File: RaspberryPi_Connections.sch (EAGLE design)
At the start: 4 parts

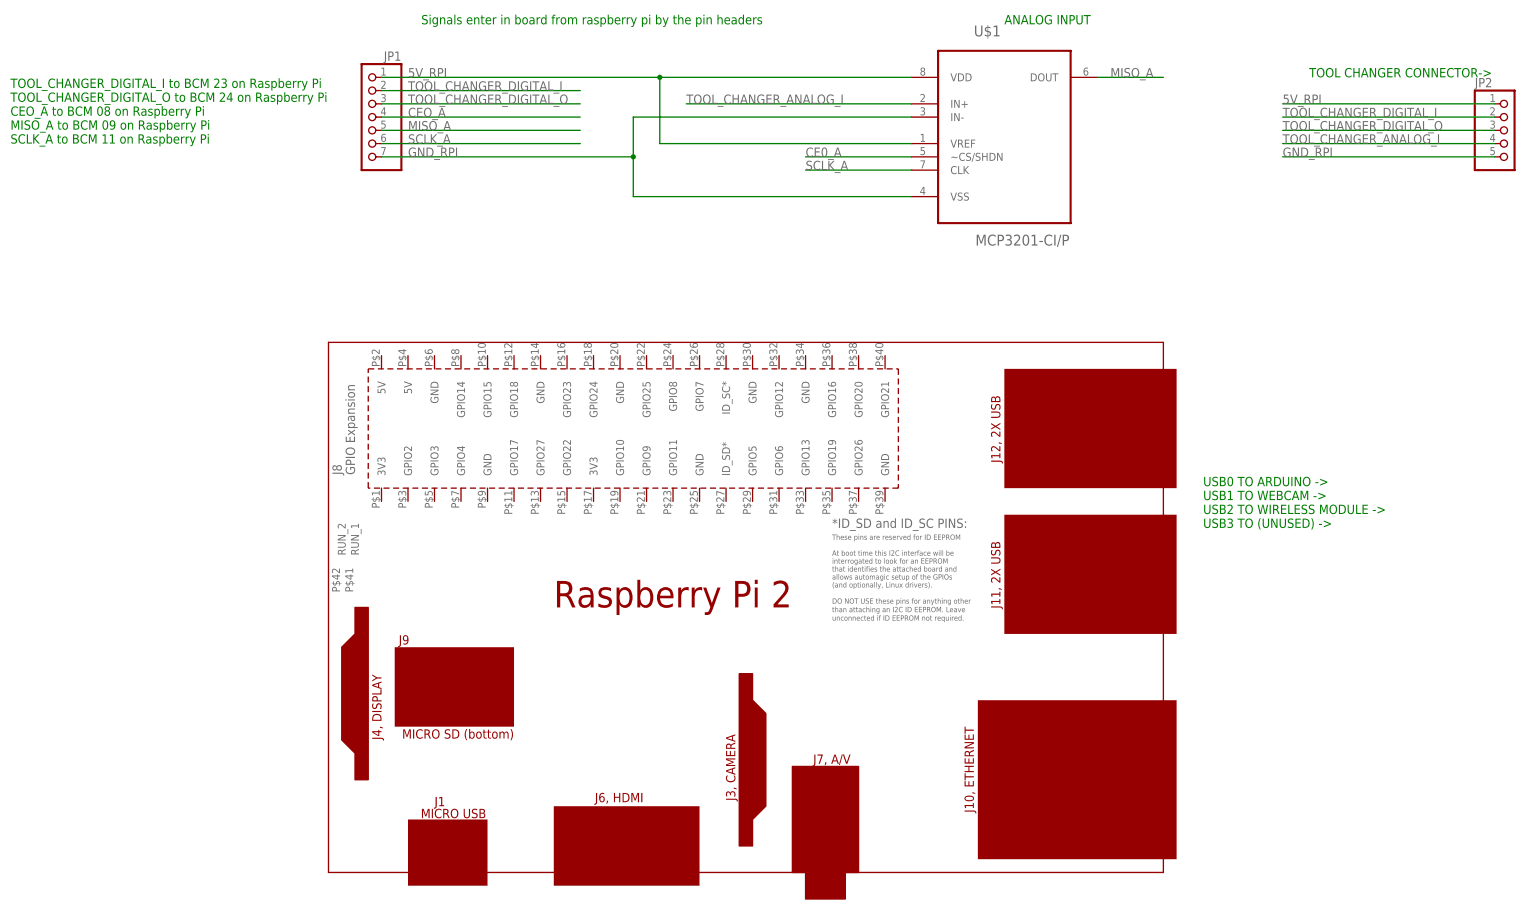
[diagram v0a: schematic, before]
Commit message: update
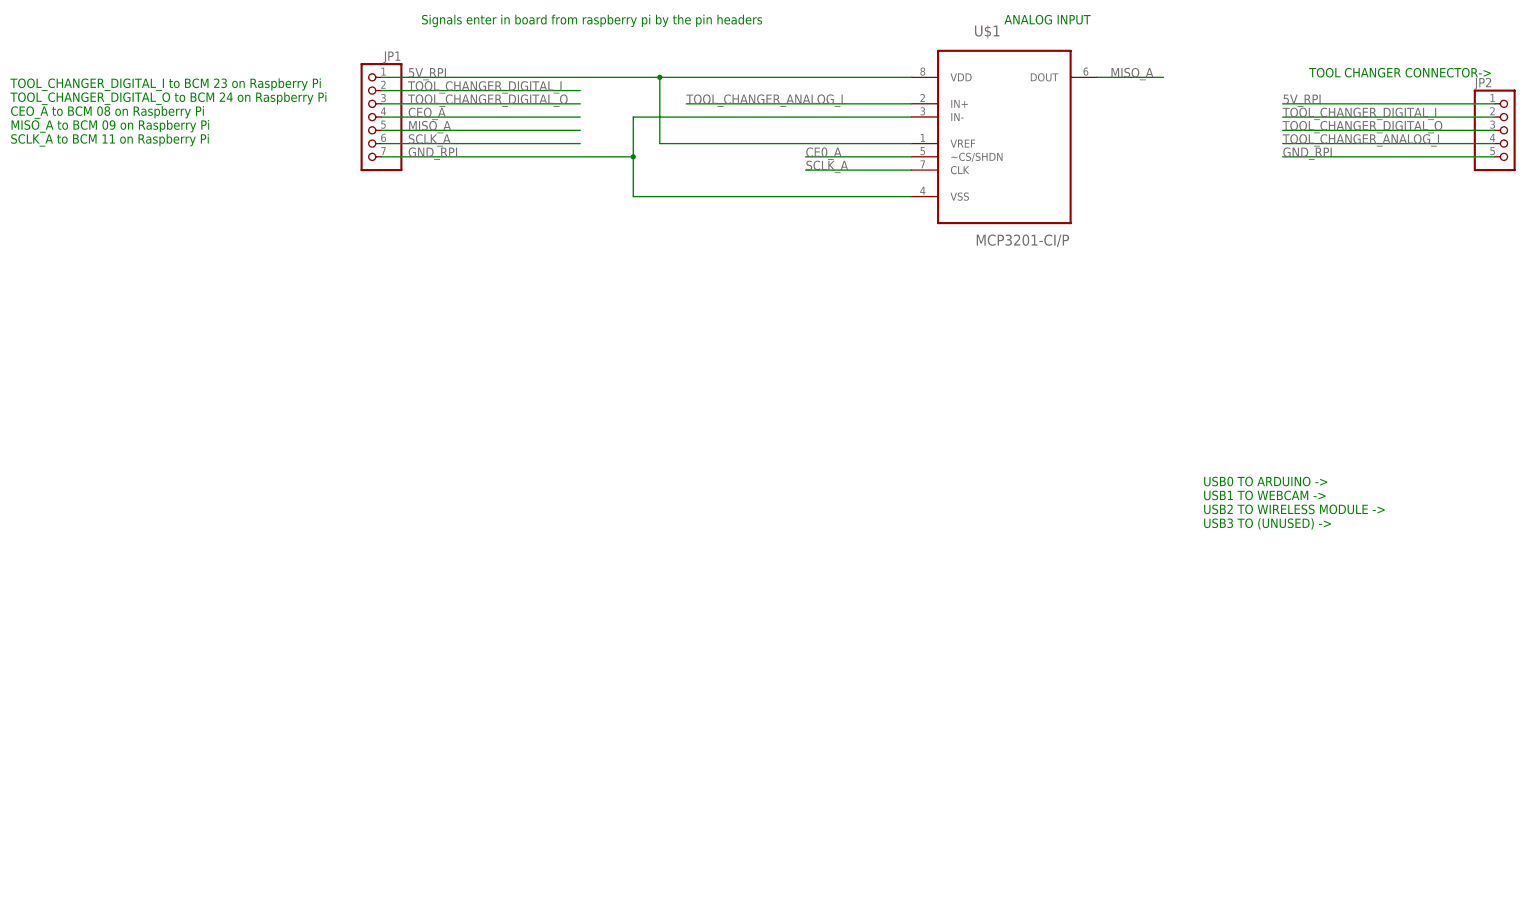
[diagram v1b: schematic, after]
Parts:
- removed PCB1: RPI2, e14_Rpi2_RevA:RPI2
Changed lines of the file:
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@@
 </classes>
 <parts>
-<part name="PCB1" library="e14_Rpi2_RevA" deviceset="RPI2" device=""/>
 <part name="JP2" library="pinhead" library_urn="urn:adsk.eagle:library:325" deviceset="PINHD-1X5" device="" package3d_urn="urn:adsk.eagle:package:22469/2"/>
 <part name="JP1" library="pinhead" library_urn="urn:adsk.eagle:library:325" deviceset="PINHD-1X7" device="" package3d_urn="urn:adsk.eagle:package:22477/2"/>
@@
 </plain>
 <instances>
-<instance part="PCB1" gate="G$1" x="10.16" y="78.74" smashed="yes"/>
 <instance part="JP2" gate="A" x="236.22" y="220.98" smashed="yes">
 <attribute name="NAME" x="229.87" y="229.235" size="1.778" layer="95"/>

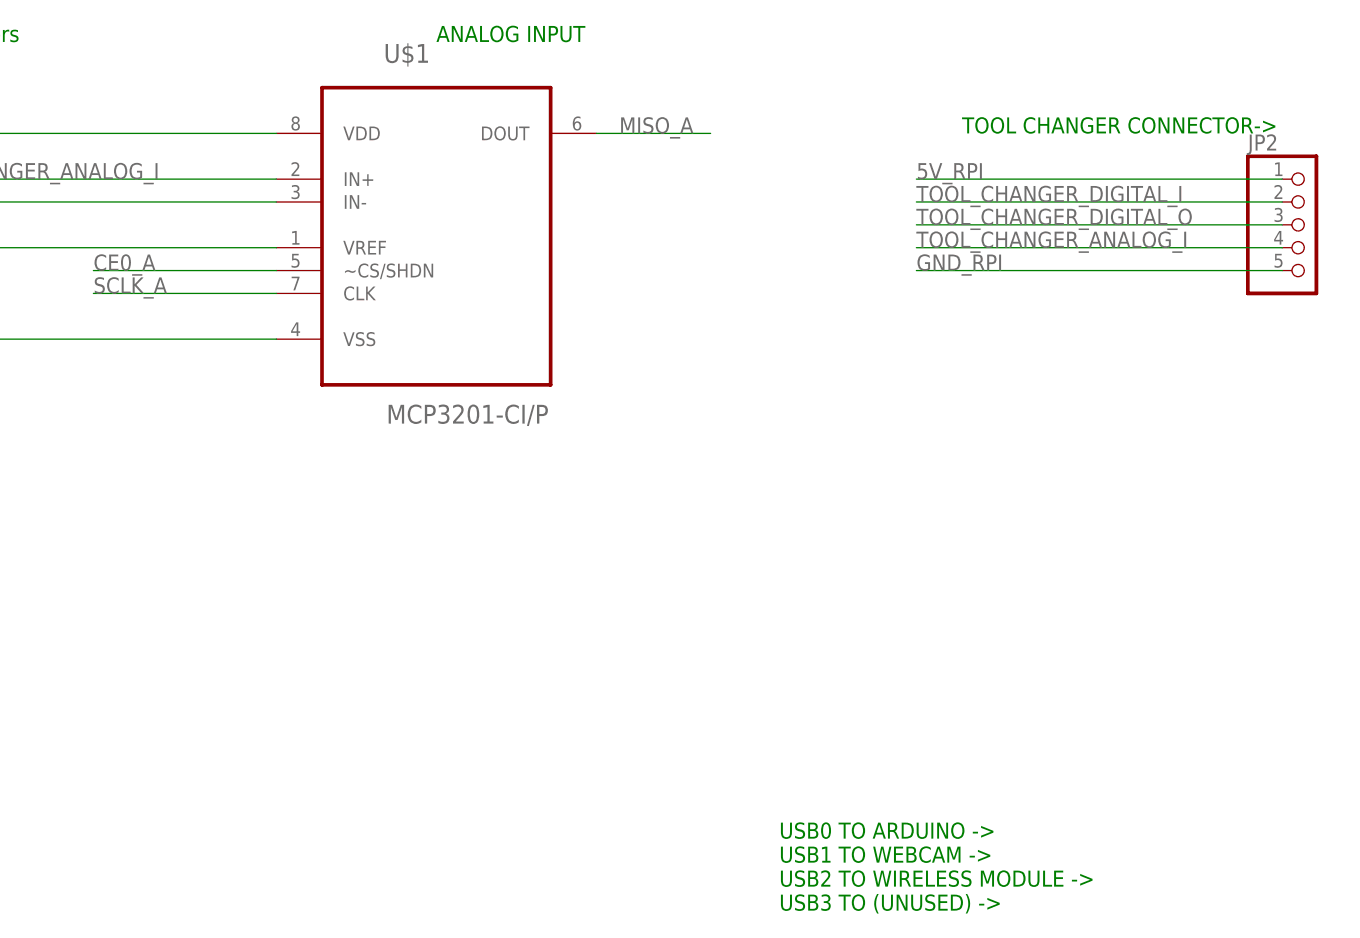
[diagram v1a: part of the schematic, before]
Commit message: update
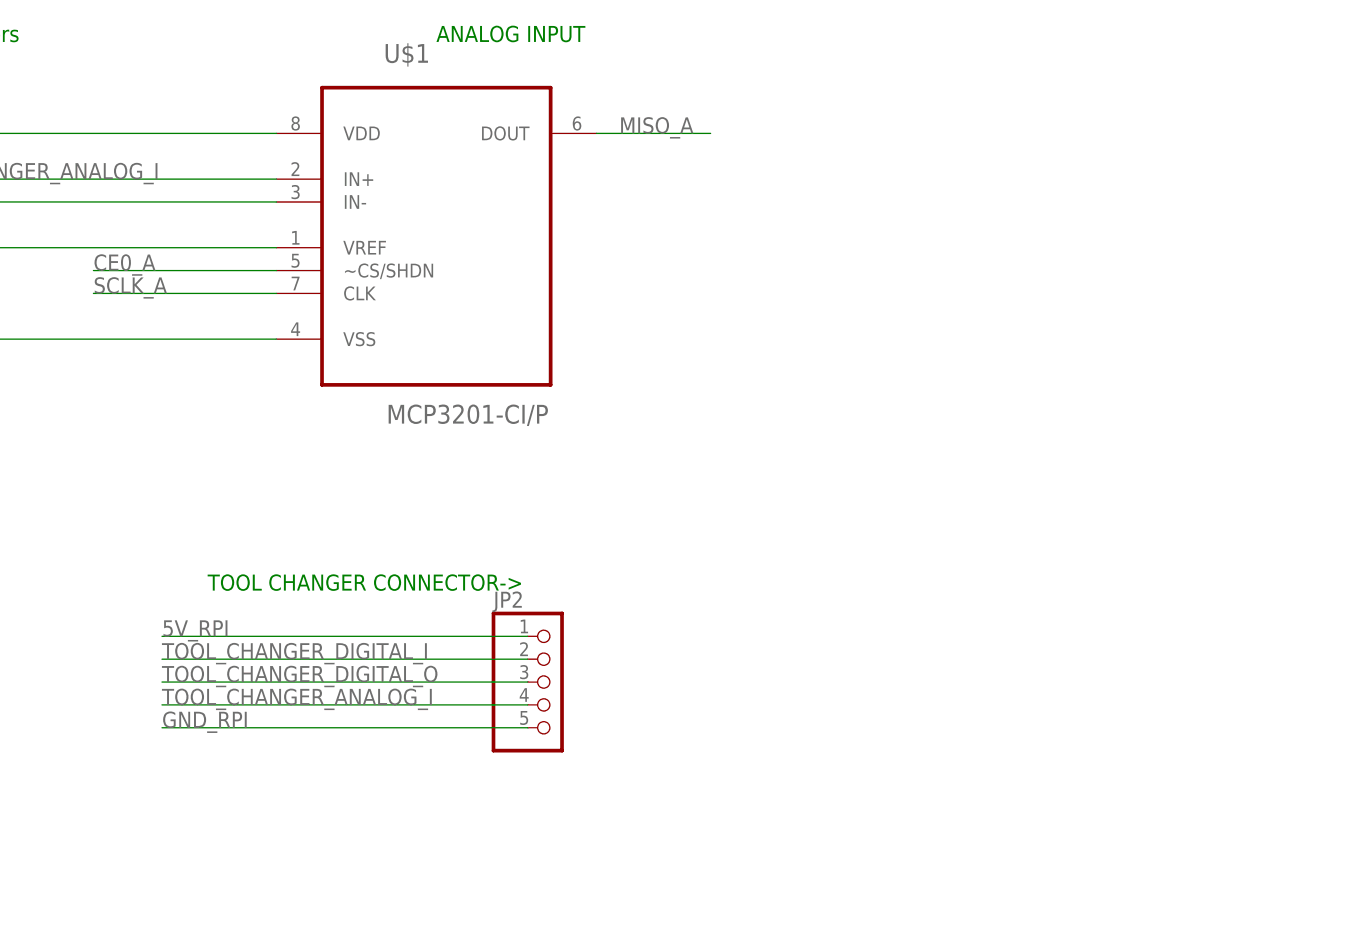
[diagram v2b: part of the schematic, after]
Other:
- note removed: "USB0 TO ARDUINO -> USB1 TO WEBCAM -> USB2 TO WIRELESS MODULE -> USB3 TO (UNUSED) ->"
- moved on the sheet: JP2
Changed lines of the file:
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@@
 <sheet>
 <plain>
-<text x="177.8" y="144.78" size="1.778" layer="91">USB0 TO ARDUINO -&gt;
-USB1 TO WEBCAM -&gt;
-USB2 TO WIRELESS MODULE -&gt;
-USB3 TO (UNUSED) -&gt;</text>
-<text x="198.12" y="231.14" size="1.778" layer="91">TOOL CHANGER CONNECTOR-&gt;</text>
+<text x="114.3" y="180.34" size="1.778" layer="91">TOOL CHANGER CONNECTOR-&gt;</text>
 <text x="139.7" y="241.3" size="1.778" layer="91">ANALOG INPUT</text>
 <text x="27.94" y="241.3" size="1.778" layer="91">Signals enter in board from raspberry pi by the pin headers</text>
@@
 </plain>
 <instances>
-<instance part="JP2" gate="A" x="236.22" y="220.98" smashed="yes">
-<attribute name="NAME" x="229.87" y="229.235" size="1.778" layer="95"/>
-<attribute name="VALUE" x="229.87" y="210.82" size="1.778" layer="96"/>
+<instance part="JP2" gate="A" x="152.4" y="170.18" smashed="yes">
+<attribute name="NAME" x="146.05" y="178.435" size="1.778" layer="95"/>
+<attribute name="VALUE" x="146.05" y="160.02" size="1.778" layer="96"/>
 </instance>
 <instance part="JP1" gate="A" x="17.78" y="223.52" smashed="yes" rot="MR0">
@@
 </segment>
 <segment>
-<wire x1="233.68" y1="226.06" x2="193.04" y2="226.06" width="0.1524" layer="91"/>
-<label x="193.04" y="226.06" size="1.778" layer="95"/>
+<wire x1="149.86" y1="175.26" x2="109.22" y2="175.26" width="0.1524" layer="91"/>
+<label x="109.22" y="175.26" size="1.778" layer="95"/>
 <pinref part="JP2" gate="A" pin="1"/>
 </segment>
@@
 </segment>
 <segment>
-<wire x1="233.68" y1="215.9" x2="193.04" y2="215.9" width="0.1524" layer="91"/>
-<label x="193.04" y="215.9" size="1.778" layer="95"/>
+<wire x1="149.86" y1="165.1" x2="109.22" y2="165.1" width="0.1524" layer="91"/>
+<label x="109.22" y="165.1" size="1.778" layer="95"/>
 <pinref part="JP2" gate="A" pin="5"/>
 </segment>
@@
 </segment>
 <segment>
-<wire x1="233.68" y1="218.44" x2="193.04" y2="218.44" width="0.1524" layer="91"/>
-<label x="193.04" y="218.44" size="1.778" layer="95"/>
+<wire x1="149.86" y1="167.64" x2="109.22" y2="167.64" width="0.1524" layer="91"/>
+<label x="109.22" y="167.64" size="1.778" layer="95"/>
 <pinref part="JP2" gate="A" pin="4"/>
 </segment>
@@
 <net name="TOOL_CHANGER_DIGITAL_O" class="0">
 <segment>
-<wire x1="233.68" y1="220.98" x2="193.04" y2="220.98" width="0.1524" layer="91"/>
-<label x="193.04" y="220.98" size="1.778" layer="95"/>
+<wire x1="149.86" y1="170.18" x2="109.22" y2="170.18" width="0.1524" layer="91"/>
+<label x="109.22" y="170.18" size="1.778" layer="95"/>
 <pinref part="JP2" gate="A" pin="3"/>
 </segment>
@@
 <net name="TOOL_CHANGER_DIGITAL_I" class="0">
 <segment>
-<wire x1="233.68" y1="223.52" x2="193.04" y2="223.52" width="0.1524" layer="91"/>
-<label x="193.04" y="223.52" size="1.778" layer="95"/>
+<wire x1="149.86" y1="172.72" x2="109.22" y2="172.72" width="0.1524" layer="91"/>
+<label x="109.22" y="172.72" size="1.778" layer="95"/>
 <pinref part="JP2" gate="A" pin="2"/>
 </segment>
